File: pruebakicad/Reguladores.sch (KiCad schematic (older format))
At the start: 9 parts, among them J6 Conn_01x02, U1 TLV1117-33, U2 TLV1117-50

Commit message: asss
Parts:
- J6: symbol Connector_Generic:Conn_01x02 -> Connector:Barrel_Jack
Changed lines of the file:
@@
 	5750 4600 5750 4750
 $Comp
-L Connector_Generic:Conn_01x02 J6
+L Connector:Barrel_Jack J6
 U 1 1 60E48AF7
 P 3350 3200

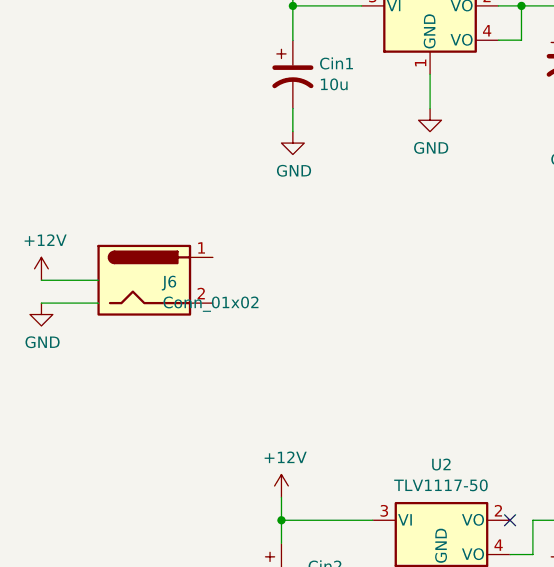
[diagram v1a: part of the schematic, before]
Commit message: asdsad
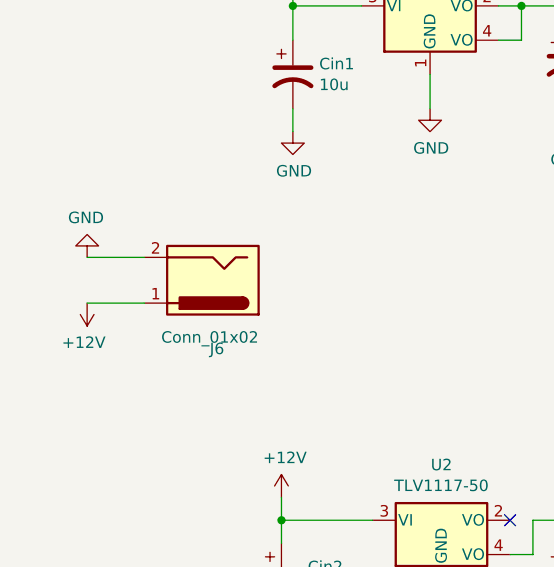
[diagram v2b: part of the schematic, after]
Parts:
- J6: footprint Connector_PinSocket_2.54mm:PinSocket_1x02_P2.54mm_Vertical -> Connector_BarrelJack:BarrelJack_CUI_PJ-063AH_Horizontal
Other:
- moved on the sheet: J6
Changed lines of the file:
@@
 L Connector:Barrel_Jack J6
 U 1 1 60E48AF7
-P 3350 3200
-F 0 "J6" H 3430 3192 50  0000 L CNN
-F 1 "Conn_01x02" H 3430 3101 50  0000 L CNN
-F 2 "Connector_PinSocket_2.54mm:PinSocket_1x02_P2.54mm_Vertical" H 3350 3200 50  0001 C CNN
-F 3 "~" H 3350 3200 50  0001 C CNN
-	1    3350 3200
-	1    0    0    -1
+P 3650 3200
+F 0 "J6" H 3600 3500 50  0000 L CNN
+F 1 "Conn_01x02" H 3450 3450 50  0000 L CNN
+F 2 "Connector_BarrelJack:BarrelJack_CUI_PJ-063AH_Horizontal" H 3650 3200 50  0001 C CNN
+F 3 "~" H 3650 3200 50  0001 C CNN
+	1    3650 3200
+	-1   0    0    1
 $EndComp
 Wire Wire Line
-	3150 3200 2900 3200
-Wire Wire Line
-	3150 3300 2900 3300
+	3350 3300 3100 3300
 $Comp
 L power:+12V #PWR?
 U 1 1 60E4A1A7
-P 2900 3200
+P 3100 3300
 AR Path="/60E4A1A7" Ref="#PWR?"  Part="1"
 AR Path="/608889A3/60E4A1A7" Ref="#PWR0140"  Part="1"
-F 0 "#PWR0140" H 2900 3050 50  0001 C CNN
-F 1 "+12V" H 2915 3373 50  0000 C CNN
-F 2 "" H 2900 3200 50  0001 C CNN
-F 3 "" H 2900 3200 50  0001 C CNN
-	1    2900 3200
-	1    0    0    -1
+F 0 "#PWR0140" H 3100 3150 50  0001 C CNN
+F 1 "+12V" H 3115 3473 50  0000 C CNN
+F 2 "" H 3100 3300 50  0001 C CNN
+F 3 "" H 3100 3300 50  0001 C CNN
+	1    3100 3300
+	-1   0    0    1
 $EndComp
 $Comp
 L power:GND #PWR?
 U 1 1 60E4A59F
-P 2900 3300
+P 3100 3100
 AR Path="/60E4A59F" Ref="#PWR?"  Part="1"
 AR Path="/608889A3/60E4A59F" Ref="#PWR0142"  Part="1"
-F 0 "#PWR0142" H 2900 3050 50  0001 C CNN
-F 1 "GND" H 2905 3127 50  0000 C CNN
-F 2 "" H 2900 3300 50  0001 C CNN
-F 3 "" H 2900 3300 50  0001 C CNN
-	1    2900 3300
-	1    0    0    -1
+F 0 "#PWR0142" H 3100 2850 50  0001 C CNN
+F 1 "GND" H 3105 2927 50  0000 C CNN
+F 2 "" H 3100 3100 50  0001 C CNN
+F 3 "" H 3100 3100 50  0001 C CNN
+	1    3100 3100
+	-1   0    0    1
 $EndComp
 Wire Wire Line
@@
 Connection ~ 5000 2000
 NoConn ~ 4950 4250
+Wire Wire Line
+	3100 3100 3350 3100
 $EndSCHEMATC
